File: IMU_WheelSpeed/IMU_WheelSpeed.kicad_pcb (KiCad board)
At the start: 2 copper layers, 56.2 x 60 mm, 24 parts, among them J1 Conn_01x04_Socket, J2 CAN_IN, J3 Conn_01x03_Socket, J4 CAN_OUT, J5 PWR_IN, J6 PWR_OUT, J7 Conn_01x07_Socket, U1 PeripheralSOM, U4 TPS71518__SC70

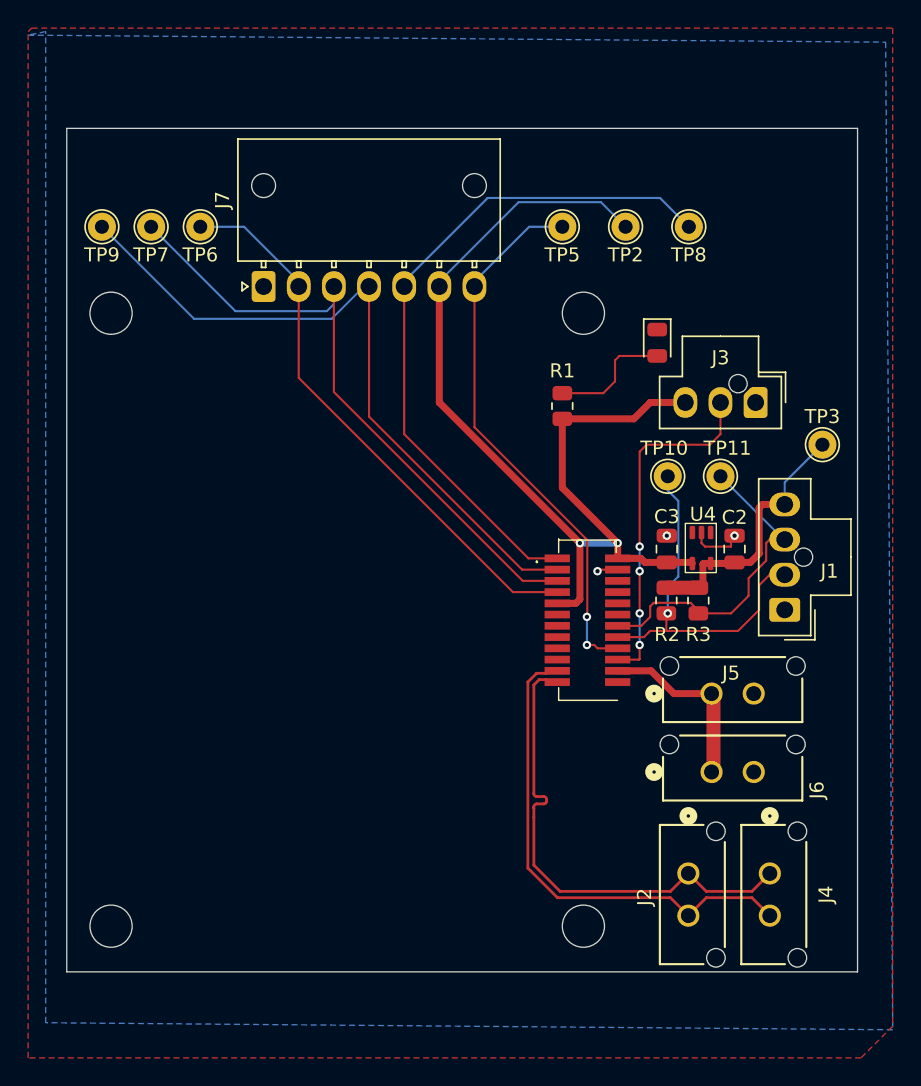
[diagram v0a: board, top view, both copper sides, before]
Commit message: made cuter and added silkscreens
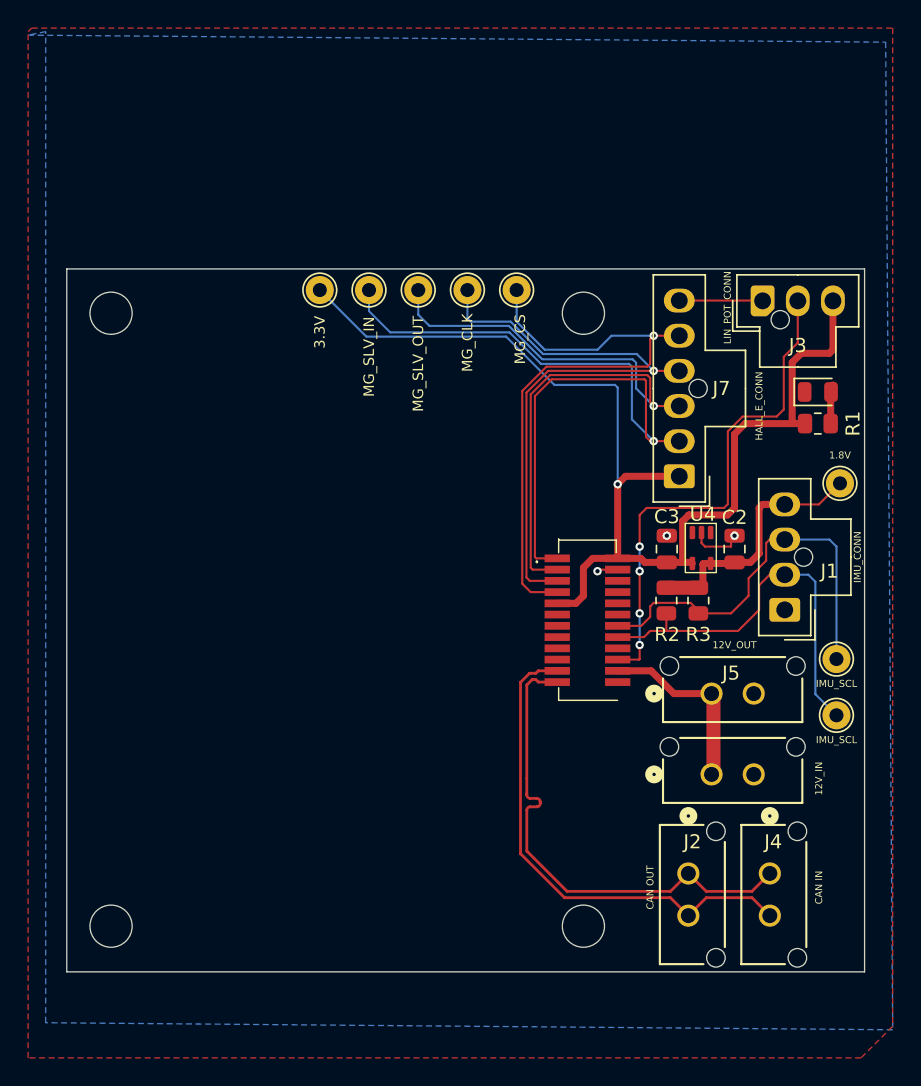
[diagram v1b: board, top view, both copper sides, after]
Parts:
- removed TP5: Mag_High, TestPoint:TestPoint_THTPad_D2.0mm_Drill1.0mm
- J7: value Conn_01x07_Socket -> Conn_01x06_Socket; footprint Connector_Molex:Molex_Nano-Fit_105313-xx07_1x07_P2.50mm_Horizontal -> Connector_Molex:Molex_Nano-Fit_105309-xx06_1x06_P2.50mm_Vertical
- moved J7 32.5 mm to (169.8, 77.5), turned to 180 degrees
- moved TP8 23.2 mm to (147.8, 64.2)
- moved TP6 22.9 mm to (158.2, 64.2)
- moved TP7 22.9 mm to (154.8, 64.2)
- moved TP9 22.9 mm to (151.2, 64.2)
- moved 3.3V 22.2 mm to (144.2, 64.2)
- moved IMU_SCL 20.8 mm to (181.0, 94.5)
- moved R1 18.2 mm to (179.7, 73.8), turned to 180 degrees
- moved IMU_SCL 15.4 mm to (181.0, 90.5)
- moved D1 11.9 mm to (179.7, 71.5), turned to 0 degrees
- moved J3 7.25 mm to (175.8, 65.0), turned to 90 degrees
- moved 1.8V 3.02 mm to (181.2, 78.0)
- moved 12V_IN 0.17 mm to (173.6, 98.4)
- renumbered TP3 to 1.8V, J6 to 12V_IN, TP2 to 3.3V, TP10 to IMU_SCL, TP11 to IMU_SCL
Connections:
- net /12V_IN renamed +12V
- J7 pad 1: GND -> /VDD_3.3V
- J7 pad 2: /MAG_CS -> /MAGSLV_Input
- J7 pad 3: /MAG_CLK -> /MAGSLV_Output
- J7 pad 4: /MAGSLV_Output -> /MAG_CLK
- J7 pad 5: /MAGSLV_Input -> /MAG_CS
- J7 pad 6: /VDD_3.3V -> GND
- U1 pad 18: /Mag_High -> unconnected-(U1-PA2(ADC)-Pad18)
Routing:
- net /Mag_High: track 39.4 -> 0.00 mm, vias 2 -> 0
- net /GPIO_1: track 24.8 -> 36.4 mm
- net /VDD_3.3V: track 73.7 -> 81.9 mm, vias 2 -> 1
- net /MAGSLV_Input: track 49.0 -> 55.8 mm, vias 0 -> 1
- net GND: track 5.32 -> 11.3 mm
- net /LTE_D1: track 8.73 -> 2.82 mm
- net /IMU_I2C_SCL: track 23.6 -> 29.0 mm
- net /MAG_CS: track 40.2 -> 43.5 mm, vias 0 -> 1
- net /MAG_CLK: track 46.3 -> 43.8 mm, vias 0 -> 1
- net /IMU_I2C_SDA: track 26.5 -> 28.7 mm, vias 1 -> 0
- net /LDO_1.8V: track 19.2 -> 18.4 mm
- net /MAGSLV_Output: track 50.3 -> 49.6 mm, vias 0 -> 1
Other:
- board size 56.2 x 60 mm -> 56.8 x 50 mm
- board text added: "12V_OUT"
- board text added: "CAN IN"
- board text added: "CAN OUT"
- board text added: "HALL_E_CONN"
- board text added: "IMU_CONN"
- board text added: "LIN_POT_CONN"
- board text added: "MG_CLK"
- board text added: "MG_CS"
- board text added: "MG_SLV_IN"
- board text added: "MG_SLV_OUT"
